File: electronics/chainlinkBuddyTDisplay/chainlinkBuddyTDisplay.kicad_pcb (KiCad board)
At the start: 2 copper layers, 74.9 x 40.6 mm, 7 parts, among them J1 Output, J2 Screw_Terminal_01x03, U1 TTGO_TDisplay

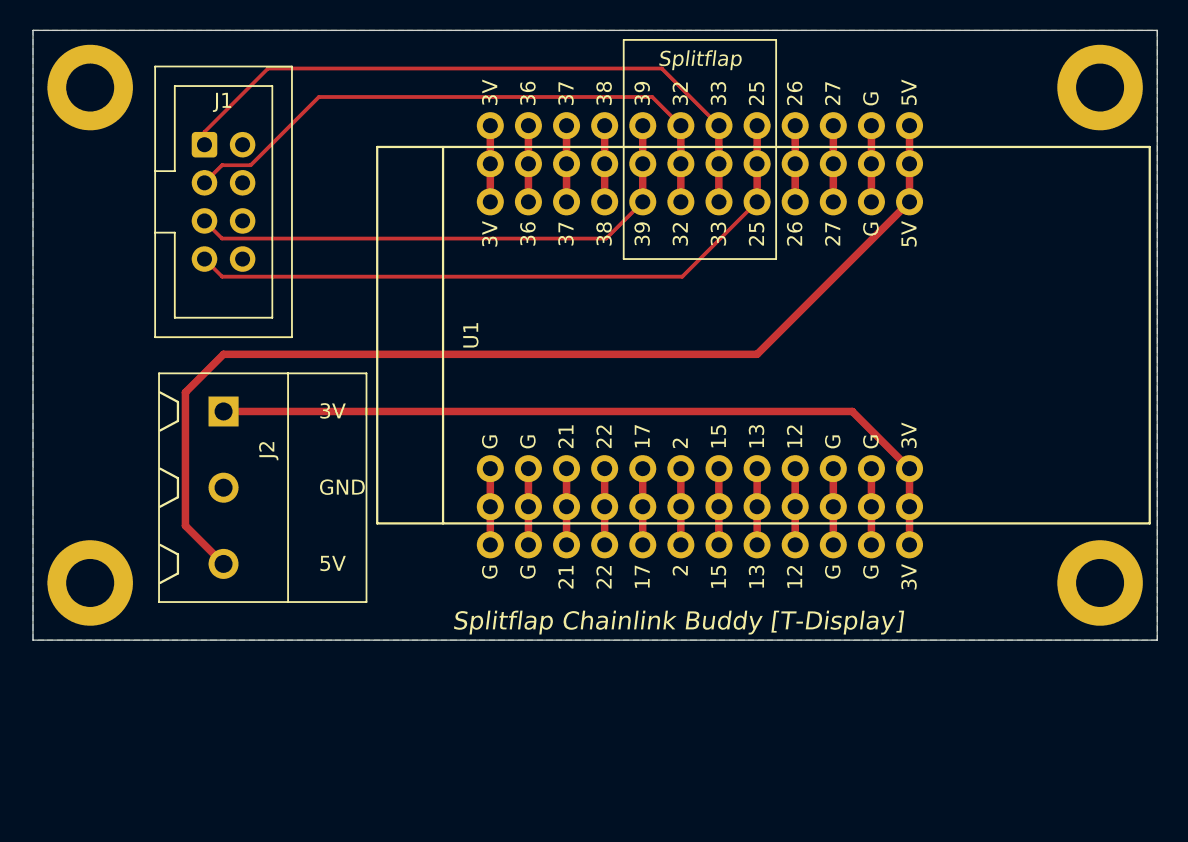
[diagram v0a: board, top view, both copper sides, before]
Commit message: Chainlink Buddy T-Display prep
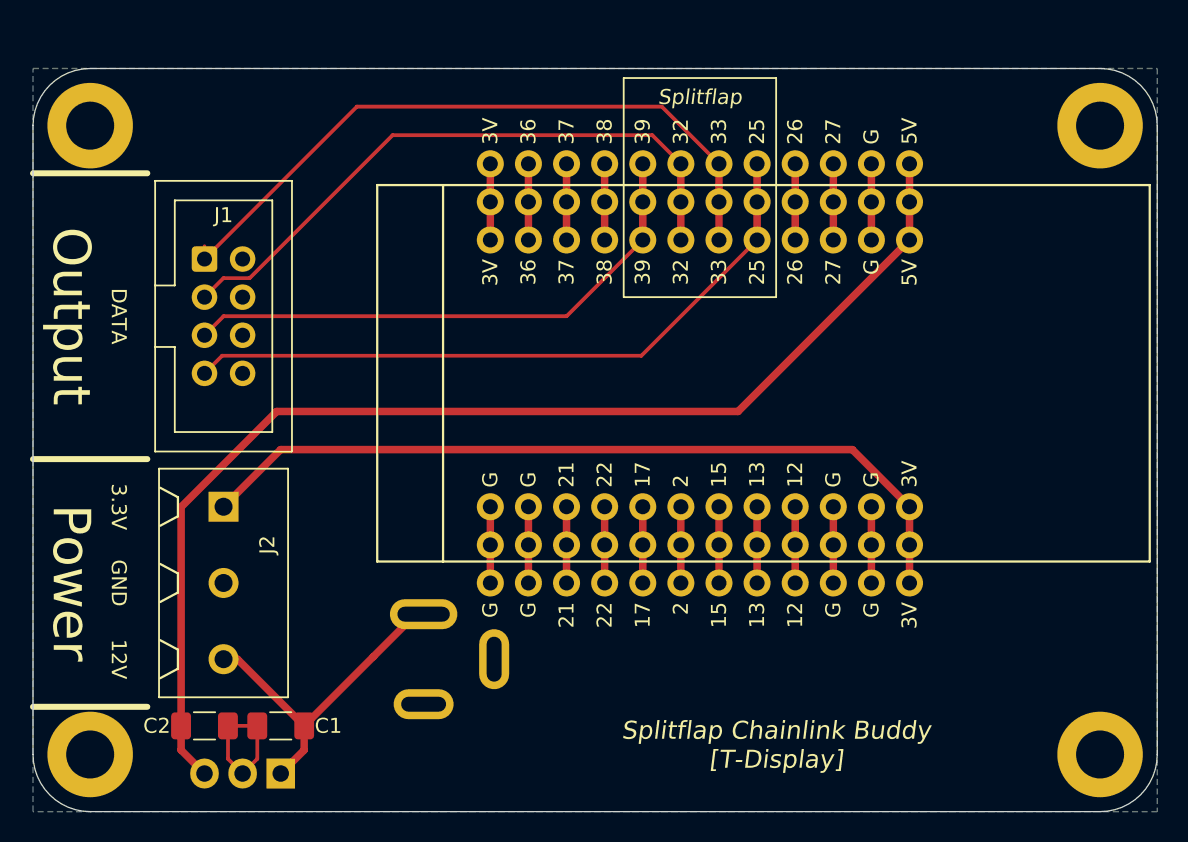
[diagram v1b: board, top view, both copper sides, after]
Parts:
- added C1: 10uF, Capacitor_SMD:C_1206_3216Metric_Pad1.33x1.80mm_HandSolder, F.Cu at (80.0, 107.3)
- added C2: 22uF, Capacitor_SMD:C_1206_3216Metric_Pad1.33x1.80mm_HandSolder, F.Cu at (74.9, 107.3)
- added J3: Barrel_Jack_Switch, PJ-202A:PJ-202A, F.Cu at (89.5, 102.9)
- added U2: LM7805_TO220, ModifiedSymbols:TO-220-3_Vertical, F.Cu at (80.0, 110.5)
- added Z1: polarity label, Symbol:Symbol_Barrel_Polarity, B.Cu at (89.5, 110.5)
- moved H3 11.4 mm to (134.6, 109.2)
- moved H4 11.4 mm to (67.3, 109.2)
- moved J1 7.62 mm to (74.9, 76.2)
- moved J2 6.35 mm to (76.2, 92.7)
- moved H1 2.54 mm to (67.3, 67.3)
- moved H2 2.54 mm to (134.6, 67.3)
- moved U1 2.54 mm to (94.0, 95.2)
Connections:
- J2 pad 3: +5V -> +12V
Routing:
- net +12V: track 0.00 -> 22.1 mm
- net GND: track 25.4 -> 34.5 mm
- net +5V: track 71.1 -> 79.4 mm
- net /CLOCK: track 43.6 -> 46.0 mm
- net /MOTOR_DATA: track 40.0 -> 42.1 mm
- net +3V3: track 52.4 -> 54.0 mm
- net /LATCH: track 44.5 -> 45.6 mm
- net /SENSOR_DATA: track 35.8 -> 36.9 mm
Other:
- board size 74.9 x 40.6 mm -> 74.9 x 49.5 mm
- board text added: "+"
- board text added: "-"
- board text added: "12V"
- board text added: "12V In"
- board text added: "3.3V"
- board text added: "5V Out"
- board text added: "Clock"
- board text added: "DATA"
- board text added: "DATE: YYYY-MM-DD COMMIT: deadbeef"
- board text added: "Latch"
- board text added: "Motor data"
- board text added: "Optional: - Install barrel jack to provide 12V motor power. - Install regulator + C1 + C2 to power ESP32 from 12V motor power."
- board text added: "Output"
- board text added: "Power"
- board text added: "Sensor data"
- board text removed: "3V"
- board text removed: "5V"
